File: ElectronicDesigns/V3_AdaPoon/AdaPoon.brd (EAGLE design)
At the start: 27.6 x 10.2 mm, 7 parts

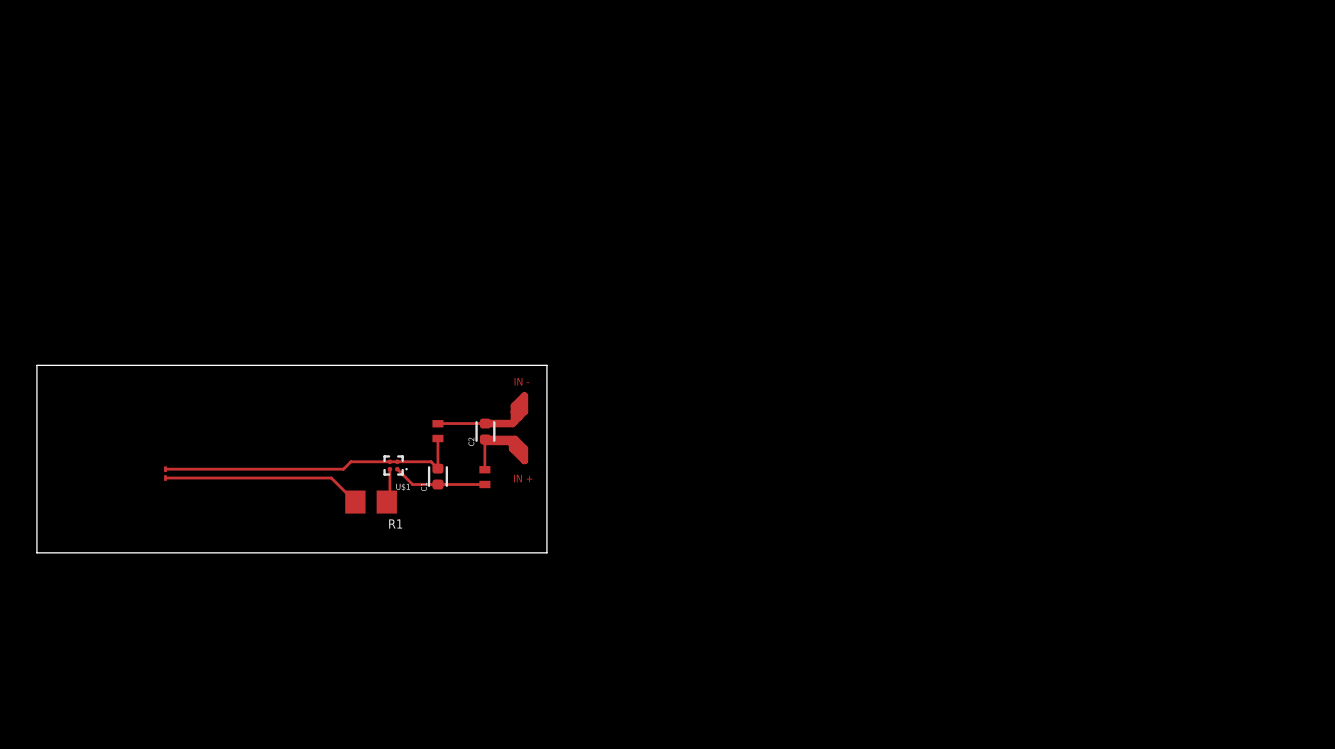
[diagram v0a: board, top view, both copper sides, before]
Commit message: Update gerbers
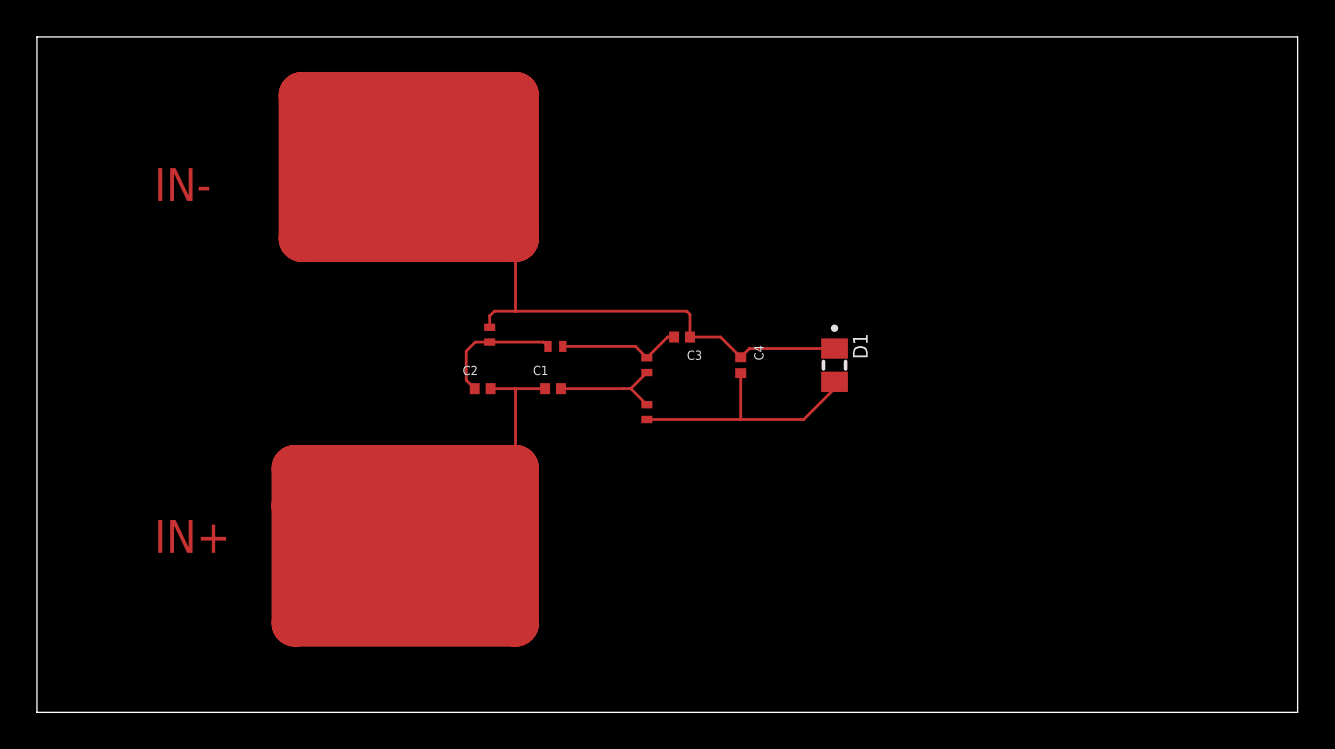
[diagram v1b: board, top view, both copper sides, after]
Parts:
- removed R1: CRCW06033K30FKEA, CRCW06033K30FKEA:RESC1608X55
- added C3, C4: 04025A100DAT2A, 04025A100DAT2A:CAPC1005X56N
- added D1: SML-LX0805SIC-TR, SML-LX0805SIC-TR:LEDC2012X120N
- C1, C2: value AMK105BJ225MV-F -> 04025A100DAT2A; device AMK105BJ225MV-F:CAPC1005X55N -> 04025A100DAT2A:CAPC1005X56N
- U$1: value BGA4C4 -> SCHOTTKY0402; device LOD_BGA4C40P2X2_84X84X60N:BGA4C40P2X2_84X84X60N -> Schottki_0402:0402_MURATA
- U$4: value CREE-TR2227 -> SCHOTTKY0402; device CREE-TR2227:CREE-TR2227 -> Schottki_0402:0402_MURATA
- moved U$4 26.3 mm to (33.0, 7.62), turned to 270 degrees
- moved U$3 11.9 mm to (33.0, 10.2), turned to 270 degrees
- moved U$1 8.79 mm to (24.5, 11.8), turned to 270 degrees
- moved U$2 8.04 mm to (28.1, 11.2), turned to 0 degrees
- moved C1 7.84 mm to (27.9, 8.89), turned to 0 degrees
- moved C2 2.32 mm to (24.1, 8.89), turned to 0 degrees
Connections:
- removed net GND: C1.2, U$1.B1, U$1.B2, U$3.P$1, U$4.P$2
- removed net N$2: R1.2, U$4.P$1
- new net N$3: C1.2, U$3.P$2, U$4.P$1
- new net N$5: C4.2, D1.A, U$4.P$2
- net IN+: now also C1.1, C2.2; no longer C2.1, U$2.P$1
- net IN-: now also C3.1, C4.1, D1.C, U$1.P$1; no longer C2.2, U$3.P$2
- net N$1: now also C2.1, U$1.P$2, U$2.P$1; no longer R1.1, U$1.A2
- net N$4: now also C3.2, U$3.P$1; no longer C1.1, U$1.A1
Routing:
- net IN-: track 8.55 -> 94.7 mm
- net IN+: track 7.81 -> 80.9 mm
- net GND: track 16.7 -> 0.00 mm
- net N$5: track 0.00 -> 13.7 mm
- net N$2: track 10.8 -> 0.00 mm
- net N$3: track 0.00 -> 6.24 mm
- net N$1: track 1.85 -> 6.95 mm
- net N$4: track 5.08 -> 6.75 mm
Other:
- board size 27.6 x 10.2 mm -> 68.2 x 36.6 mm
- board text added: "IN+"
- board text added: "IN-"
- board text removed: "IN +"
- board text removed: "IN -"
